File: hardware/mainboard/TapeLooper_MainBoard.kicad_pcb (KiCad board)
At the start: 2 copper layers, 119.5 x 106.5 mm, 242 parts, among them J1 Micro_SD_Card, J10 VOL_B, J11 PITCH_C, J12 PITCH_D, J13 VOL_C, J14 VOL_D, J2 Conn_02x05_Odd_Even, J3 AUDIO_IN_L, J4 AUDIO_IN_R, J5 AUDIO_OUT_L, J6 AUDIO_OUT_R, J7 PITCH_A, J8 PITCH_B, J9 VOL_A, SW1 BTTN_LOAD, SW10 BTTN_PLAY_B, SW11 BTTN_PLAY_C, SW12 BTTN_PLAY_D, SW2 BTTN_DIRECTION, SW3 BTTN_SAVE, SW4 BTTN_REC, SW5 BTTN_SPEED_A, SW6 BTTN_SPEED_B, SW7 BTTN_SPEED_C, SW8 BTTN_SPEED_D, SW9 BTTN_PLAY_A, U1 DAISY_SEED, U10 AZ1117-2.5, U11 AZ1117-3.3, U2 EC4SAW-24S05N, U3 AZ1117-5.0, U4 TL074, U5 PCA9685PW, U6 PCA9685PW, U7 PCA9685PW, U8 MAX11300_TQFP, U9 MAX11300_TQFP

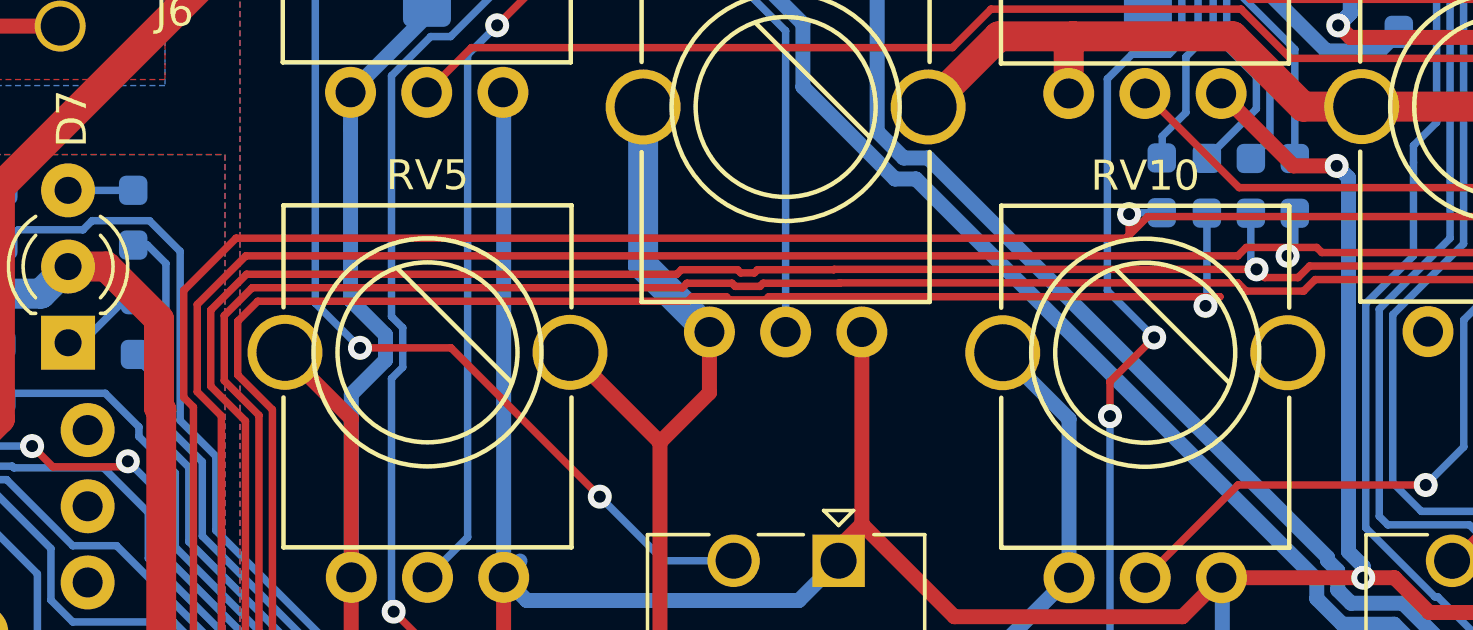
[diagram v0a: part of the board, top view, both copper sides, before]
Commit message: hardware: update schematics & add BOM
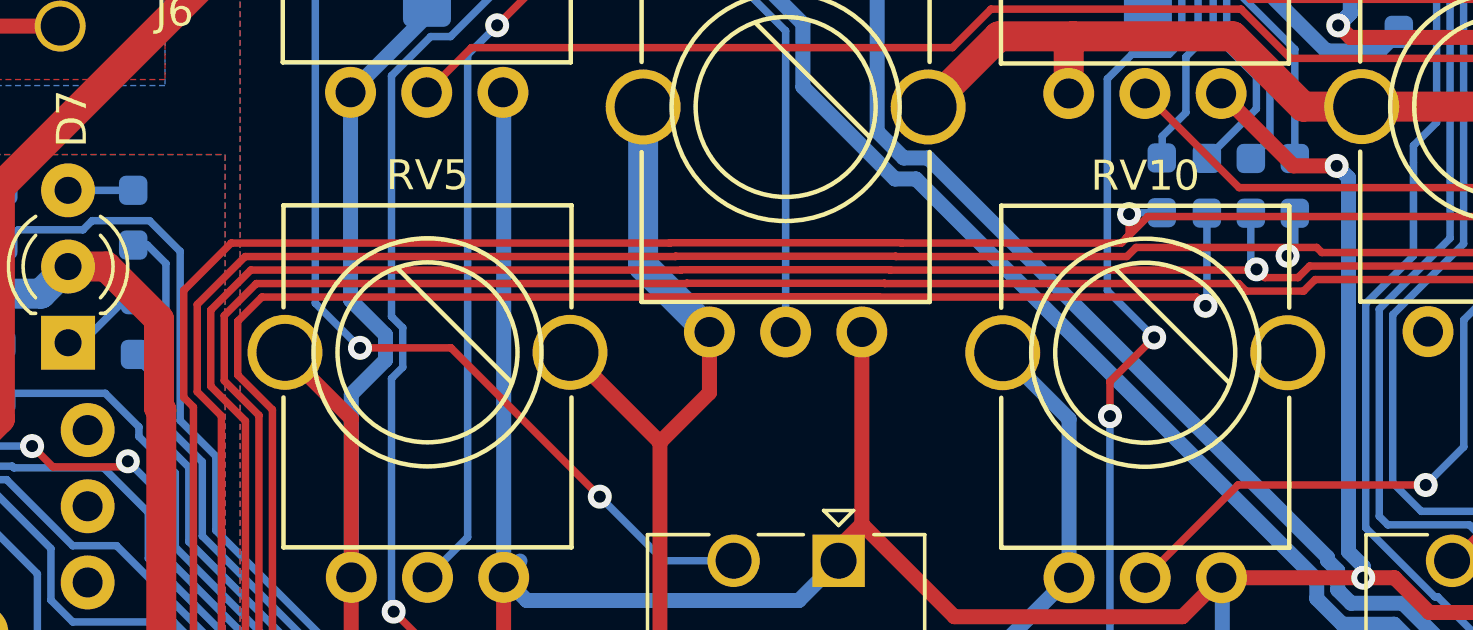
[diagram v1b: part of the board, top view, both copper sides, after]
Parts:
- D10: value LED_DIRECTION -> LED_RED_GREEN_CA
- D11: value LED_REC -> LED_RED_GREEN_CA
- D12: value LED_SPEED_+2_A -> LED_RED_GREEN_CA
- D13: value LED_SPEED_+2_C -> LED_RED_GREEN_CA
- D14: value LED_SPEED_+1_A -> LED_RED_GREEN_CA
- D15: value LED_SPEED_+1_C -> LED_RED_GREEN_CA
- D16: value LED_SPEED_-1_A -> LED_RED_GREEN_CA
- D17: value LED_SPEED_-1_C -> LED_RED_GREEN_CA
- D18: value LED_SPEED_-2_A -> LED_RED_GREEN_CA
- D19: value LED_SPEED_-2_C -> LED_RED_GREEN_CA
- D20: value LED_SPEED_+2_B -> LED_RED_GREEN_CA
- D21: value LED_SPEED_+2_D -> LED_RED_GREEN_CA
- D22: value LED_SPEED_+1_B -> LED_RED_GREEN_CA
- D23: value LED_SPEED_+1_D -> LED_RED_GREEN_CA
- D24: value LED_SPEED_-1_B -> LED_RED_GREEN_CA
- D25: value LED_SPEED_-1_D -> LED_RED_GREEN_CA
- D26: value LED_SPEED_-2_B -> LED_RED_GREEN_CA
- D27: value LED_SPEED_-2_D -> LED_RED_GREEN_CA
- D4: value LED_IN_L -> LED_RED_GREEN_CA
- D5: value LED_IN_R -> LED_RED_GREEN_CA
- D6: value LED_OUT_L -> LED_RED_GREEN_CA
- D7: value LED_OUT_R -> LED_RED_GREEN_CA
- D8: value LED_LOAD -> LED_RED_GREEN_CA
- D9: value LED_SAVE -> LED_RED_GREEN_CA
- J10: value VOL_B -> PJ398SM
- J11: value PITCH_C -> PJ398SM
- J12: value PITCH_D -> PJ398SM
- J13: value VOL_C -> PJ398SM
- J14: value VOL_D -> PJ398SM
- J3: value AUDIO_IN_L -> PJ398SM
- J4: value AUDIO_IN_R -> PJ398SM
- J5: value AUDIO_OUT_L -> PJ398SM
- J6: value AUDIO_OUT_R -> PJ398SM
- J7: value PITCH_A -> PJ398SM
- J8: value PITCH_B -> PJ398SM
- J9: value VOL_A -> PJ398SM
- R21, R22, R23, R26, R27, R28, R29, R30, R31, R32, R33, R34, R35, R36, R37, R38, R39, R40, R41, R42, R43, R44, R45, R46, R47, R48, R49, R50, R51, R52, R53, R54, R55, R56, R57, R58, R59, R60, R61, R62, R63, R64, R65, R66, R67, R68, R69, R70: value Rled -> 330
- SW1: value BTTN_LOAD -> TL1105SPF250Q
- SW10: value BTTN_PLAY_B -> D6R90F1LFS
- SW11: value BTTN_PLAY_C -> D6R90F1LFS
- SW12: value BTTN_PLAY_D -> D6R90F1LFS
- SW2: value BTTN_DIRECTION -> TL1105SPF250Q
- SW3: value BTTN_SAVE -> TL1105SPF250Q
- SW4: value BTTN_REC -> D6R40F1LFS
- SW5: value BTTN_SPEED_A -> C&K 7105SYCQE
- SW6: value BTTN_SPEED_B -> C&K 7105SYCQE
- SW7: value BTTN_SPEED_C -> C&K 7105SYCQE
- SW8: value BTTN_SPEED_D -> C&K 7105SYCQE
- SW9: value BTTN_PLAY_A -> D6R90F1LFS
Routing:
- net SPI_CS_AB: track 57.1 -> 56.1 mm
